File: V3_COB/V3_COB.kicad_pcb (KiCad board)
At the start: 4 copper layers, 16 x 16 mm, 3 parts, among them J101 Conn_02x35_Counter_Clockwise_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, J102 Conn_2Rows-76Pins

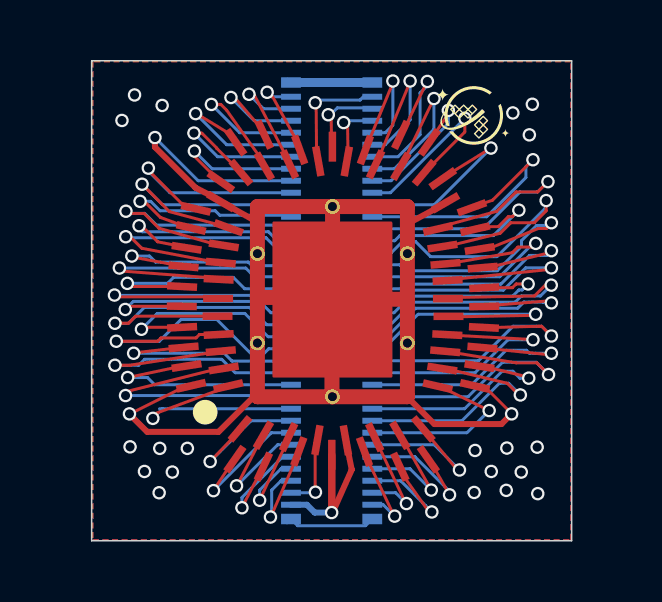
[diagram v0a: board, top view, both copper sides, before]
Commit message: XP update in V3_COB (clean up works)
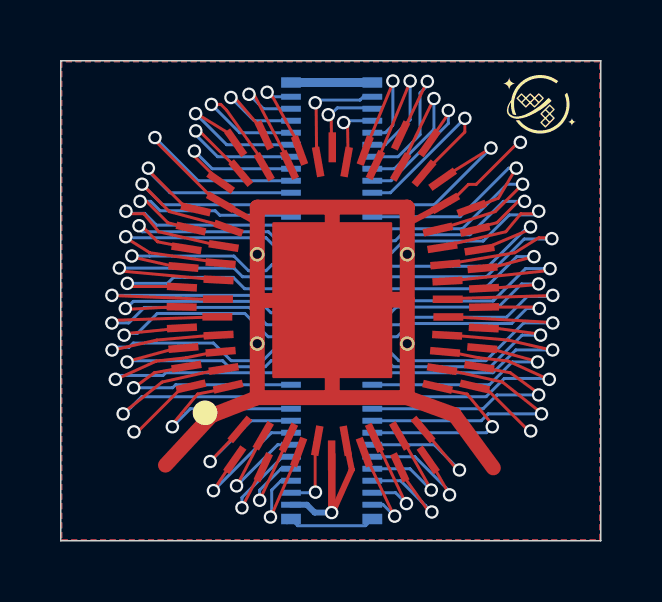
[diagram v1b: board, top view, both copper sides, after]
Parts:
- removed J102: Conn_2Rows-76Pins, MOSBius_V2_CHIP:round_COB
- added J1: Conn_2Rows-76Pins, MOSBius_V2_CHIP:round_COB, F.Cu at (204.2, 63.5)
- moved G*** 2.25 mm to (211.2, 56.8)
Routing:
- net GND: track 46.7 -> 22.8 mm, vias 23 -> 4
- net /PIN 15: track 10.2 -> 6.47 mm
- net /PIN 13: track 10.1 -> 6.42 mm
- net /PIN 11: track 9.58 -> 6.14 mm
- net /PIN 56: track 8.49 -> 5.76 mm
- net /PIN 53: track 9.25 -> 6.63 mm
- net /PIN 12: track 7.82 -> 5.91 mm
- net /PIN 55: track 8.63 -> 7.02 mm
- net /PIN 41: track 7.76 -> 6.17 mm
- net /PIN 52: track 7.36 -> 5.84 mm
- net /PIN 46: track 6.46 -> 7.82 mm
- net /PIN 48: track 7.11 -> 5.94 mm
- net /PIN 44: track 7.13 -> 6.13 mm
- net /PIN 14: track 6.91 -> 6.07 mm
- net /PIN 45: track 5.92 -> 6.70 mm
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- added copper zone on In2.Cu, net GND
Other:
- board size 16 x 16 mm -> 18 x 16 mm
- board text removed: "Allocated Space For Passives"
